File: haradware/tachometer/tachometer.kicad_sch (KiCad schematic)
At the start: 5 parts, among them U1 RP2040, U2 LM393

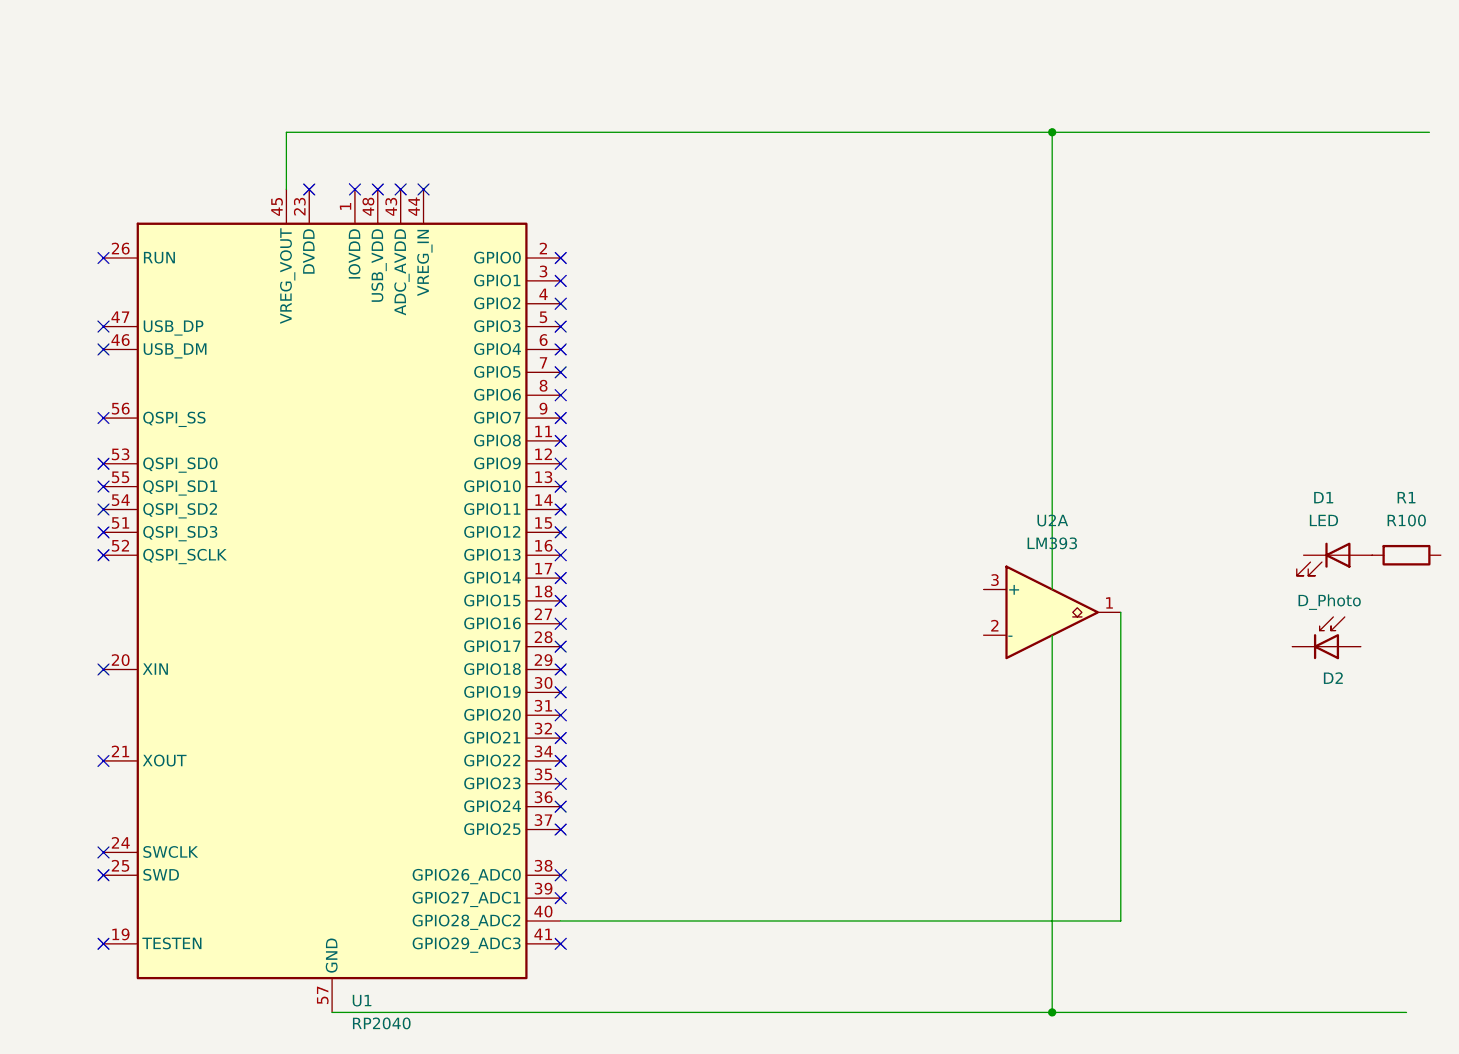
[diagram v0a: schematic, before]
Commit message: KiCad編集
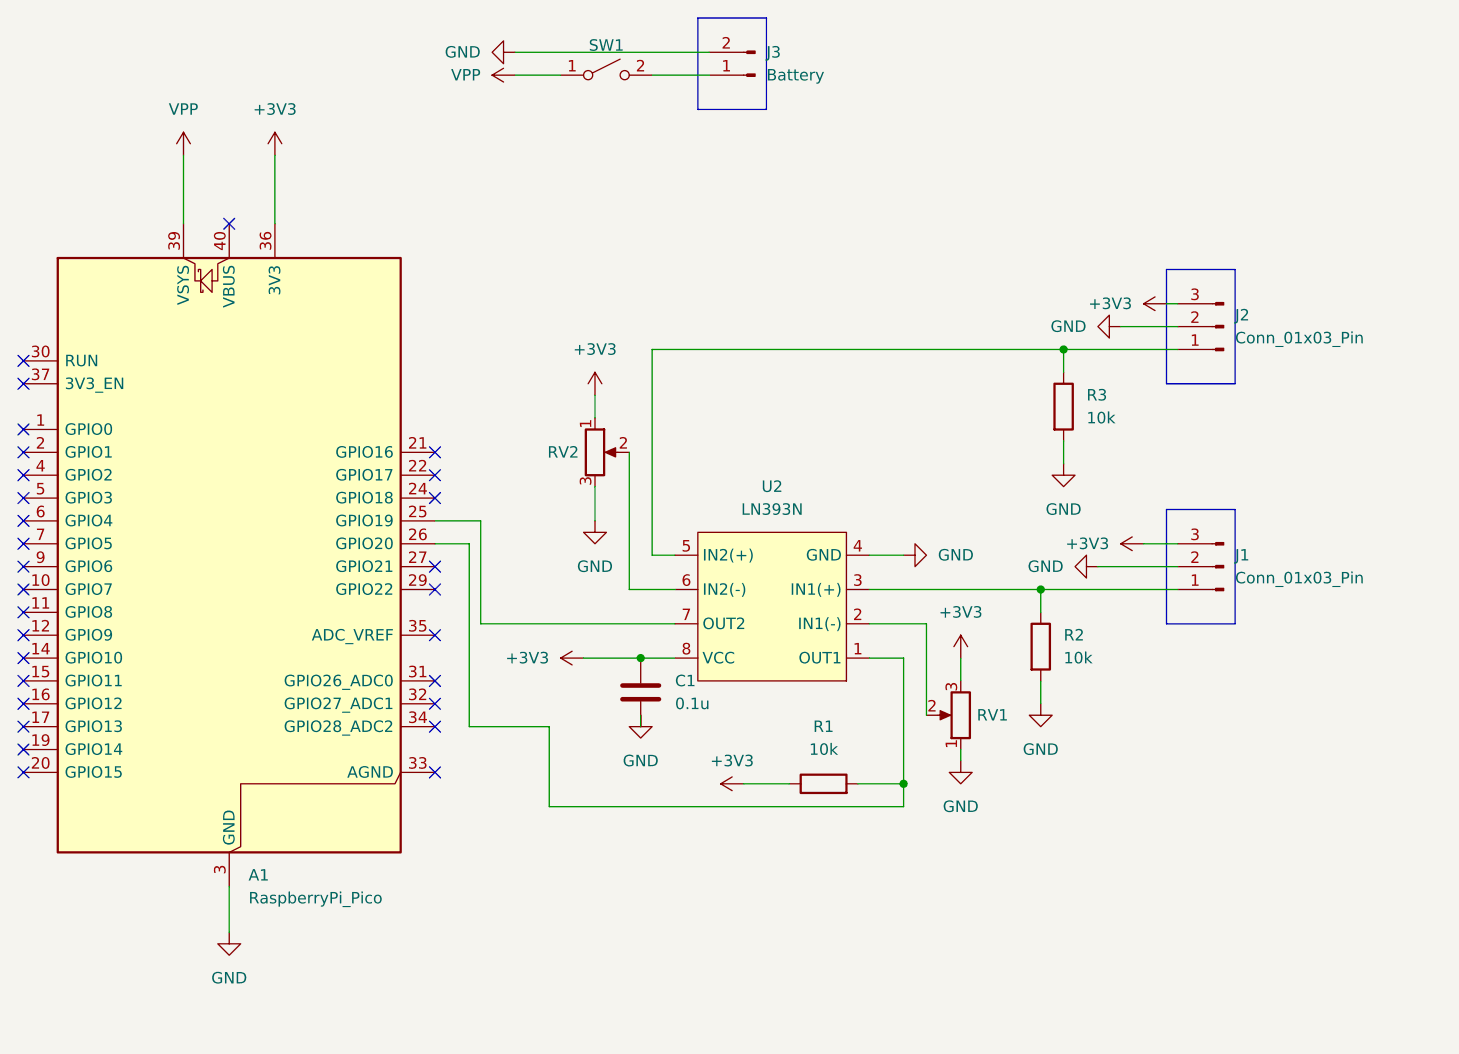
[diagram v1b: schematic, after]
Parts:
- removed D1: LED, symbol Device:LED
- removed D2: D_Photo, symbol Device:D_Photo
- removed U1: RP2040, Package_DFN_QFN:QFN-56-1EP_7x7mm_P0.4mm_EP3.2x3.2mm, symbol MCU_RaspberryPi:RP2040
- removed U2: LM393, symbol Comparator:LM393
- added A1: RaspberryPi_Pico, Module:RaspberryPi_Pico_Common_Unspecified, symbol MCU_Module:RaspberryPi_Pico
- added C1: 0.1u, Capacitor_THT:C_Axial_L5.1mm_D3.1mm_P10.00mm_Horizontal, symbol Device:C
- added J1, J2: Conn_01x03_Pin, Connector_JST:JST_PH_B3B-PH-K_1x03_P2.00mm_Vertical, symbol Connector:Conn_01x03_Pin
- added J3: Battery, Connector_JST:JST_PH_B2B-PH-K_1x02_P2.00mm_Vertical, symbol Connector:Conn_01x02_Pin
- added R2, R3: 10k, Resistor_THT:R_Axial_DIN0207_L6.3mm_D2.5mm_P7.62mm_Horizontal, symbol Device:R
- added RV1, RV2: R_Potentiometer, Potentiometer_THT:Potentiometer_Bourns_3296P_Horizontal, symbol Device:R_Potentiometer
- added SW1: SW_SPST, Button_Switch_THT:SW_Slide-03_Wuerth-WS-SLTV_10x2.5x6.4_P2.54mm, symbol Switch:SW_SPST
- added U2: LN393N, Package_DIP:CERDIP-8_W7.62mm_SideBrazed, symbol New_Library:LN393
- R1: value R100 -> 10k; footprint (none) -> Resistor_THT:R_Axial_DIN0207_L6.3mm_D2.5mm_P7.62mm_Horizontal
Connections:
- net at R1.2: now also A1.26 (GPIO20), U2.1 (OUT1)
- net +3V3: now reaches R1.1
- net +3V3: now also A1.36 (3V3), C1.1, J1.3 (Pin_3), J2.3 (Pin_3), RV1.3, RV2.1, U2.8 (VCC)
- new net: RV2.2, U2.6 (IN2(-))
- new net: J3.1 (Pin_1), SW1.2 (B)
- new net: A1.25 (GPIO19), U2.7 (OUT2)
- new net: RV1.2, U2.2 (IN1(-))
- new net: J1.1 (Pin_1), R2.1, U2.3 (IN1(+))
- new net: J2.1 (Pin_1), R3.1, U2.5 (IN2(+))
- new net GND: A1.13 (GND), A1.18 (GND), A1.23 (GND), A1.28 (GND), A1.3 (GND), A1.38 (GND), A1.8 (GND), C1.2, J1.2 (Pin_2), J2.2 (Pin_2), J3.2 (Pin_2), R2.2, R3.2, RV1.1, RV2.3, U2.4 (GND)
- new net VPP: A1.39 (VSYS), SW1.1 (A)
- no-connect marks 48 -> 29
